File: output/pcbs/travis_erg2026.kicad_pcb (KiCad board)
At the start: 2 copper layers, 163.4 x 159.9 mm, 173 parts

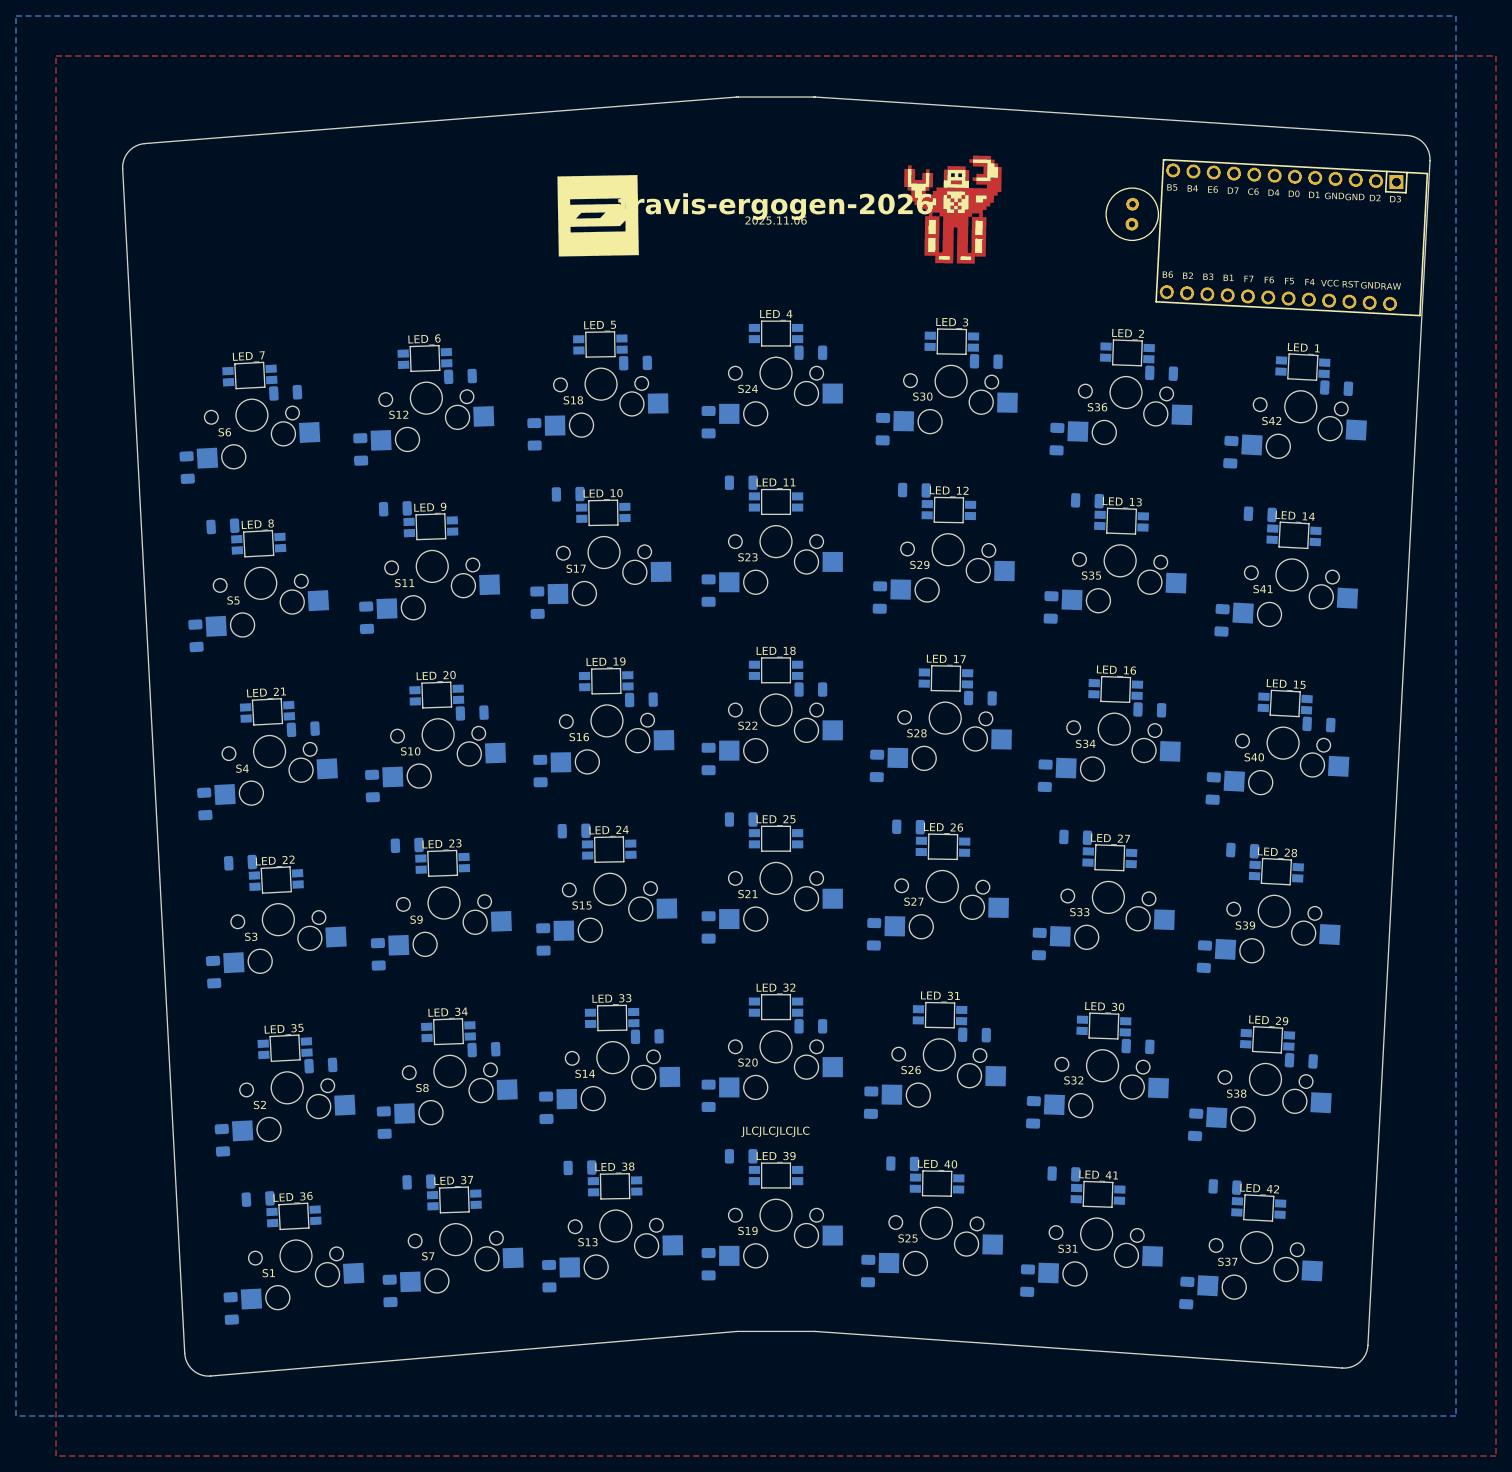
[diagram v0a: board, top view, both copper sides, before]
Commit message: updates
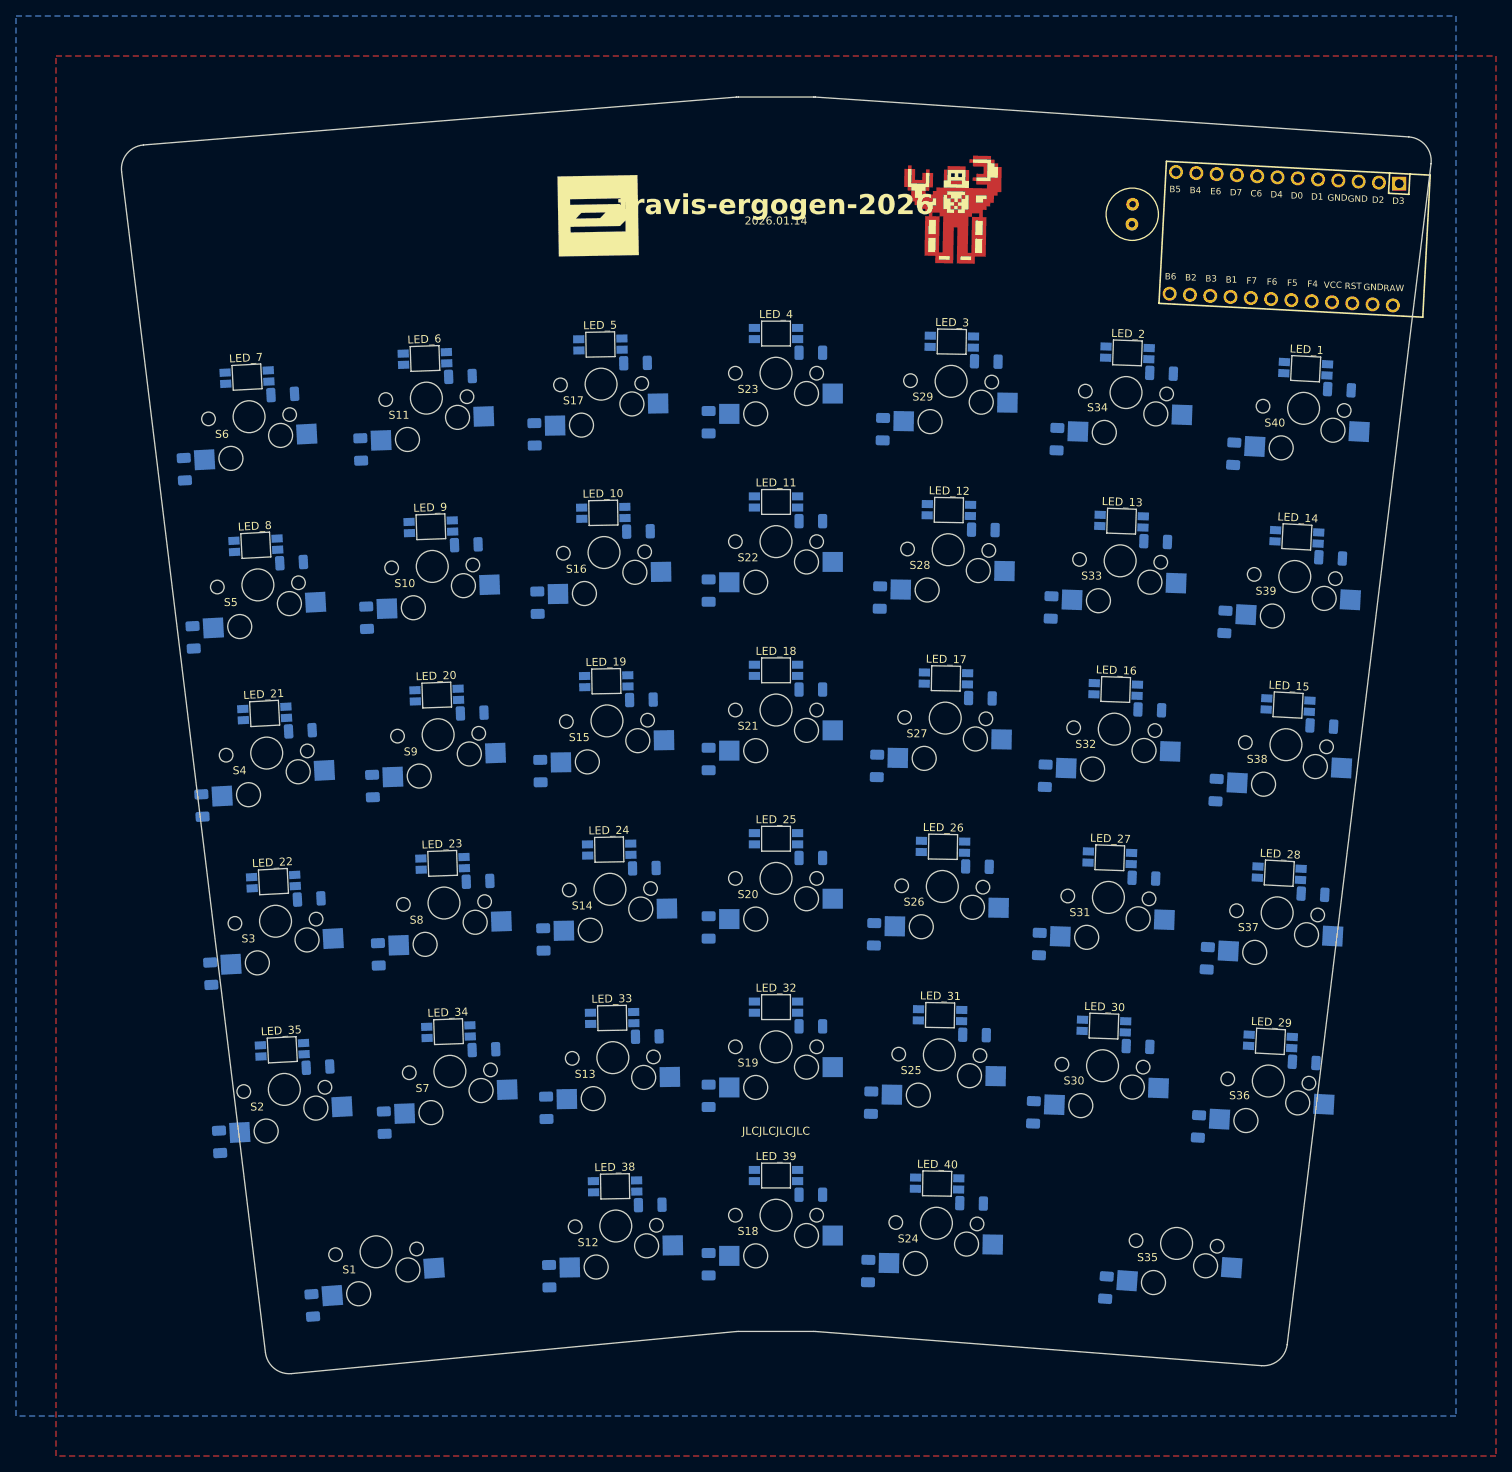
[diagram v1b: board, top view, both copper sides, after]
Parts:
- removed C40, C41, C42, C43: C_1206_3216Metric, C_1206_3216Metric
- removed D41, D42: D_1206_3216Metric, D_1206_3216Metric
- removed LED39, LED40, LED41, LED42: SK6812mini-e, travis:led_SK6812mini-e (per-key, single-side)
- removed S41, S42: Kailh MX Switch Sockets, travis:MX
- moved S24 108.1 mm to (130.1, 195.9), turned to 179 degrees
- moved D24 108.0 mm to (121.5, 201.9), turned to 89 degrees
- moved S18 106.2 mm to (110.0, 194.9), turned to 180 degrees
- moved S12 106.2 mm to (90.0, 196.3), turned to 181 degrees
- moved D12 106.0 mm to (81.7, 202.5), turned to 91 degrees
- moved D18 106.0 mm to (101.6, 201.0), turned to 90 degrees
- moved S36 87.9 mm to (171.5, 178.1), turned to 177 degrees
- moved D36 87.7 mm to (162.8, 183.8), turned to 87 degrees
- moved S30 87.6 mm to (150.8, 176.2), turned to 178 degrees
- moved D30 87.4 mm to (142.2, 182.0), turned to 88 degrees
- moved S35 85.6 mm to (160.1, 198.4), turned to 176 degrees
- moved D35 85.3 mm to (151.2, 203.9), turned to 86 degrees
- moved LED28 84.2 mm to (88.4, 107.1)
- moved LED34 84.2 mm to (131.6, 106.8)
- moved LED31 84.2 mm to (110.0, 105.7)
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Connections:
- D10 pad 1: row3 -> row4
- D10 pad 2: matrix_col1_row3 -> matrix_col1_row4
- D11 pad 1: row4 -> row5
- D11 pad 2: matrix_col1_row4 -> matrix_col1_row5
- D12 pad 1: row5 -> row0
- D12 pad 2: matrix_col1_row5 -> matrix_col2_row0
- D13 pad 1: row0 -> row1
- D13 pad 2: matrix_col2_row0 -> matrix_col2_row1
- D14 pad 1: row1 -> row2
- D14 pad 2: matrix_col2_row1 -> matrix_col2_row2
- D15 pad 1: row2 -> row3
- D15 pad 2: matrix_col2_row2 -> matrix_col2_row3
- D16 pad 1: row3 -> row4
- D16 pad 2: matrix_col2_row3 -> matrix_col2_row4
- D17 pad 1: row4 -> row5
- D17 pad 2: matrix_col2_row4 -> matrix_col2_row5
- D18 pad 1: row5 -> row0
- D18 pad 2: matrix_col2_row5 -> matrix_col3_row0
- D19 pad 1: row0 -> row1
- D19 pad 2: matrix_col3_row0 -> matrix_col3_row1
- D20 pad 1: row1 -> row2
- D20 pad 2: matrix_col3_row1 -> matrix_col3_row2
- D21 pad 1: row2 -> row3
- D21 pad 2: matrix_col3_row2 -> matrix_col3_row3
- D22 pad 1: row3 -> row4
- D22 pad 2: matrix_col3_row3 -> matrix_col3_row4
- D23 pad 1: row4 -> row5
- D23 pad 2: matrix_col3_row4 -> matrix_col3_row5
- D24 pad 1: row5 -> row0
- D24 pad 2: matrix_col3_row5 -> matrix_col4_row0
- D25 pad 1: row0 -> row1
- D25 pad 2: matrix_col4_row0 -> matrix_col4_row1
- D26 pad 1: row1 -> row2
- D26 pad 2: matrix_col4_row1 -> matrix_col4_row2
- D27 pad 1: row2 -> row3
- D27 pad 2: matrix_col4_row2 -> matrix_col4_row3
- D28 pad 1: row3 -> row4
- D28 pad 2: matrix_col4_row3 -> matrix_col4_row4
- D29 pad 1: row4 -> row5
- D29 pad 2: matrix_col4_row4 -> matrix_col4_row5
- D30 pad 1: row5 -> row1
- D30 pad 2: matrix_col4_row5 -> matrix_col5_row1
- D31 pad 1: row0 -> row2
- D31 pad 2: matrix_col5_row0 -> matrix_col5_row2
- D32 pad 1: row1 -> row3
- D32 pad 2: matrix_col5_row1 -> matrix_col5_row3
- D33 pad 1: row2 -> row4
- D33 pad 2: matrix_col5_row2 -> matrix_col5_row4
- D34 pad 1: row3 -> row5
- D34 pad 2: matrix_col5_row3 -> matrix_col5_row5
- D35 pad 1: row4 -> row0
- D35 pad 2: matrix_col5_row4 -> matrix_col6_row0
- D36 pad 1: row5 -> row1
- D36 pad 2: matrix_col5_row5 -> matrix_col6_row1
- D37 pad 1: row0 -> row2
- D37 pad 2: matrix_col6_row0 -> matrix_col6_row2
- D38 pad 1: row1 -> row3
- D38 pad 2: matrix_col6_row1 -> matrix_col6_row3
- D39 pad 1: row2 -> row4
- D39 pad 2: matrix_col6_row2 -> matrix_col6_row4
- D40 pad 1: row3 -> row5
- D40 pad 2: matrix_col6_row3 -> matrix_col6_row5
- D7 pad 1: row0 -> row1
- D7 pad 2: matrix_col1_row0 -> matrix_col1_row1
- D8 pad 1: row1 -> row2
- D8 pad 2: matrix_col1_row1 -> matrix_col1_row2
- D9 pad 1: row2 -> row3
- D9 pad 2: matrix_col1_row2 -> matrix_col1_row3
- LED22 pad 2: LED_37 -> LED_23
- LED22 pad 4: LED_36 -> LED_22
- LED23 pad 2: LED_23 -> LED_9
- LED23 pad 4: LED_22 -> LED_8
- LED24 pad 2: LED_9 -> LED_24
- LED24 pad 4: LED_8 -> LED_23
- LED25 pad 2: LED_38 -> LED_10
- LED25 pad 4: LED_37 -> LED_9
- LED26 pad 2: LED_24 -> LED_39
- LED26 pad 4: LED_23 -> LED_38
- LED27 pad 2: LED_10 -> LED_25
- LED27 pad 4: LED_9 -> LED_24
- LED28 pad 2: LED_39 -> LED_11
- LED28 pad 4: LED_38 -> LED_10
- LED29 pad 2: LED_25 -> LED_40
- LED29 pad 4: LED_24 -> LED_39
- LED30 pad 2: LED_11 -> LED_26
- LED30 pad 4: LED_10 -> LED_25
- LED31 pad 2: LED_40 -> LED_12
- LED31 pad 4: LED_39 -> LED_11
- LED32 pad 2: LED_26 -> LED_41
- LED32 pad 4: LED_25 -> LED_40
- LED33 pad 2: LED_12 -> LED_27
- LED33 pad 4: LED_11 -> LED_26
- LED34 pad 2: LED_41 -> LED_13
- LED34 pad 4: LED_40 -> LED_12
- LED35 pad 2: LED_27 -> LED_28
- LED35 pad 4: LED_26 -> LED_27
- LED36 pad 2: LED_13 -> LED_14
- LED36 pad 4: LED_12 -> LED_13
- LED37 pad 2: LED_42 -> LED_29
- LED37 pad 4: LED_41 -> LED_28
- LED38 pad 2: LED_28 -> LED_13
- LED38 pad 4: LED_27 -> LED_14
- S10 pad 2: matrix_col1_row3 -> matrix_col1_row4
- S11 pad 2: matrix_col1_row4 -> matrix_col1_row5
- S12 pad 1: col1 -> col2
- S12 pad 2: matrix_col1_row5 -> matrix_col2_row0
- S13 pad 2: matrix_col2_row0 -> matrix_col2_row1
- S14 pad 2: matrix_col2_row1 -> matrix_col2_row2
- S15 pad 2: matrix_col2_row2 -> matrix_col2_row3
- S16 pad 2: matrix_col2_row3 -> matrix_col2_row4
- S17 pad 2: matrix_col2_row4 -> matrix_col2_row5
- S18 pad 1: col2 -> col3
- S18 pad 2: matrix_col2_row5 -> matrix_col3_row0
- S19 pad 2: matrix_col3_row0 -> matrix_col3_row1
- S20 pad 2: matrix_col3_row1 -> matrix_col3_row2
- S21 pad 2: matrix_col3_row2 -> matrix_col3_row3
- S22 pad 2: matrix_col3_row3 -> matrix_col3_row4
- S23 pad 2: matrix_col3_row4 -> matrix_col3_row5
- S24 pad 1: col3 -> col4
- S24 pad 2: matrix_col3_row5 -> matrix_col4_row0
- S25 pad 2: matrix_col4_row0 -> matrix_col4_row1
- S26 pad 2: matrix_col4_row1 -> matrix_col4_row2
- S27 pad 2: matrix_col4_row2 -> matrix_col4_row3
- S28 pad 2: matrix_col4_row3 -> matrix_col4_row4
- S29 pad 2: matrix_col4_row4 -> matrix_col4_row5
- S30 pad 1: col4 -> col5
- S30 pad 2: matrix_col4_row5 -> matrix_col5_row1
- S31 pad 2: matrix_col5_row0 -> matrix_col5_row2
- S32 pad 2: matrix_col5_row1 -> matrix_col5_row3
- S33 pad 2: matrix_col5_row2 -> matrix_col5_row4
- S34 pad 2: matrix_col5_row3 -> matrix_col5_row5
- S35 pad 1: col5 -> col6
- S35 pad 2: matrix_col5_row4 -> matrix_col6_row0
- S36 pad 1: col5 -> col6
- S36 pad 2: matrix_col5_row5 -> matrix_col6_row1
- S37 pad 2: matrix_col6_row0 -> matrix_col6_row2
- S38 pad 2: matrix_col6_row1 -> matrix_col6_row3
- S39 pad 2: matrix_col6_row2 -> matrix_col6_row4
- S40 pad 2: matrix_col6_row3 -> matrix_col6_row5
- S7 pad 2: matrix_col1_row0 -> matrix_col1_row1
- S8 pad 2: matrix_col1_row1 -> matrix_col1_row2
- S9 pad 2: matrix_col1_row2 -> matrix_col1_row3
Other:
- board size 163.4 x 159.9 mm -> 163.7 x 159.6 mm
- board text added: "2026.01.14"
- board text removed: "2025.11.06"
- board text removed: "LED_36"
- board text removed: "LED_37"
- board text removed: "LED_41"
- board text removed: "LED_42"
- board text removed: "S41"
- board text removed: "S42"
